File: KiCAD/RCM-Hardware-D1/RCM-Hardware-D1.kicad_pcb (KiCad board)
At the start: 2 copper layers, 33 x 55.9 mm, 2 parts, among them U1 WeMos_D1_mini, U2 L293D

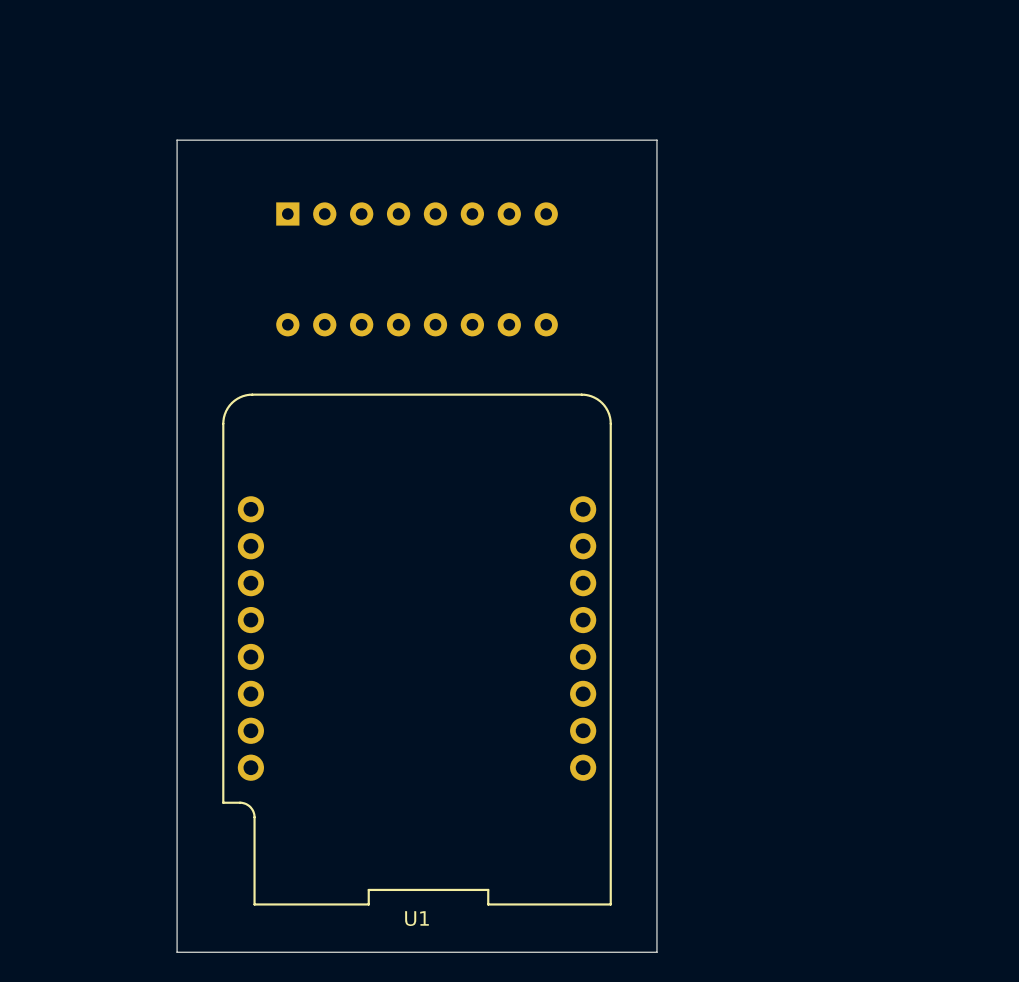
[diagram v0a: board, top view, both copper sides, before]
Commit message: set up kicad
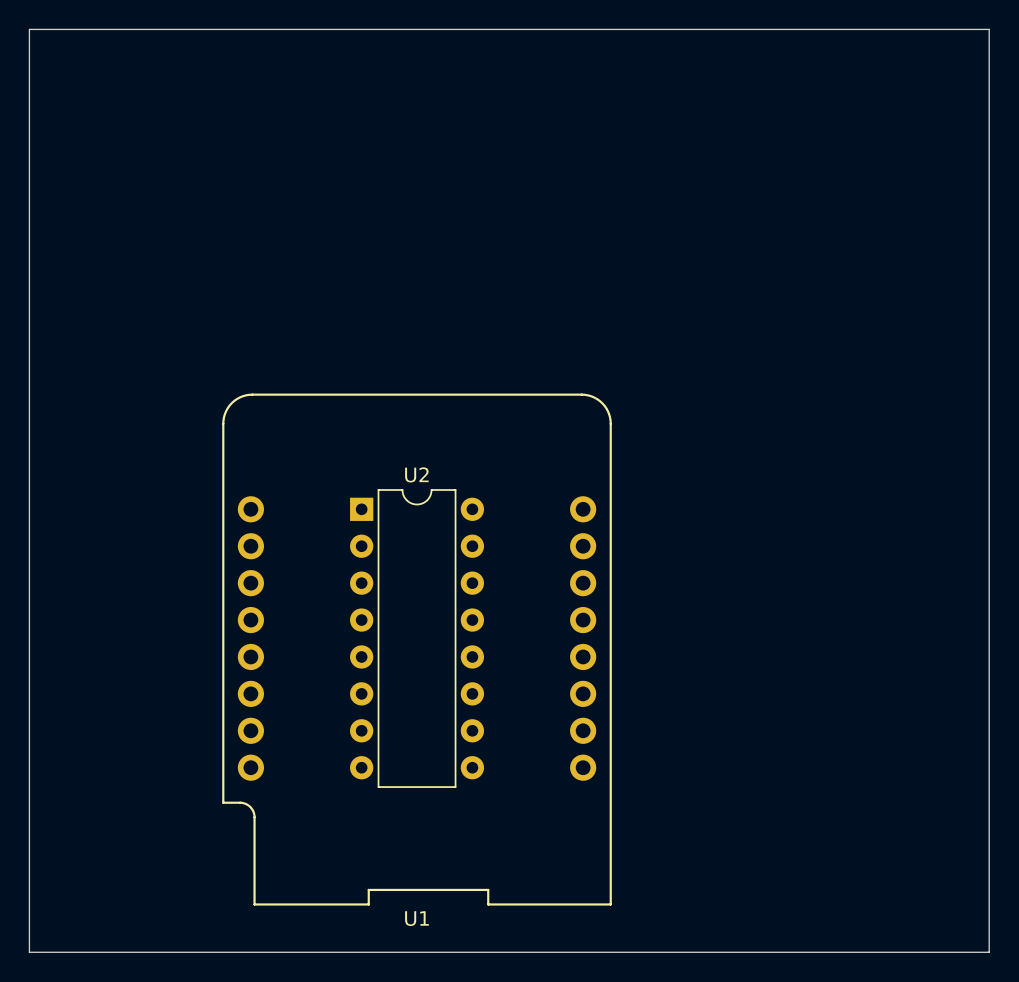
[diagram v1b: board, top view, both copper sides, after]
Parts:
- U2: moved to F.Cu
- moved U2 20.9 mm to (134.6, 76.2), turned to 0 degrees
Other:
- board size 33 x 55.9 mm -> 66 x 63.5 mm
